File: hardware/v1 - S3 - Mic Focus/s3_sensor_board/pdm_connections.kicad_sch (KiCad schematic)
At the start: 2 parts, among them U501 SHT4x

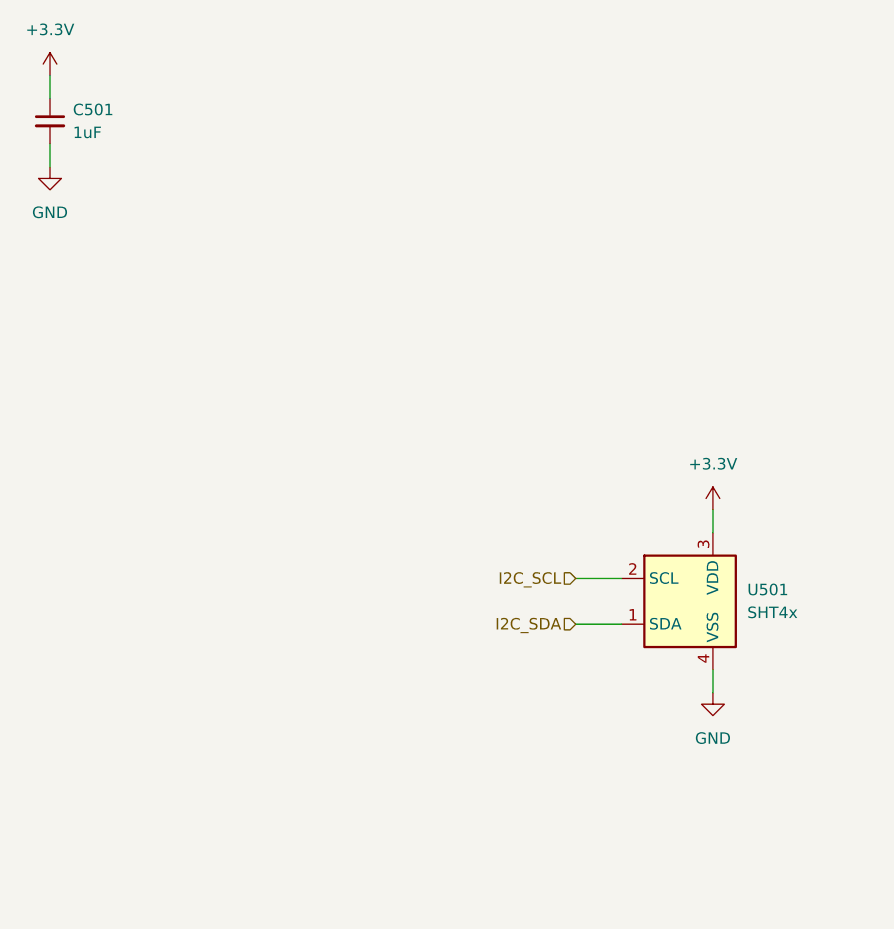
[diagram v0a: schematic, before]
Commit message: WIP
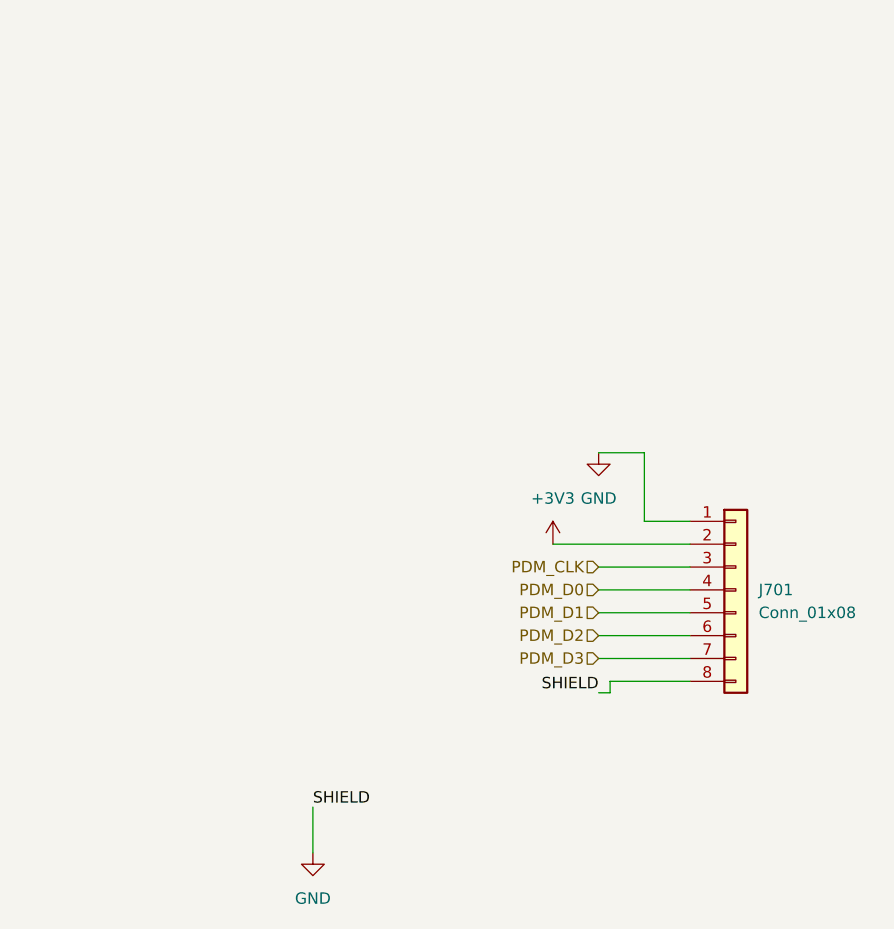
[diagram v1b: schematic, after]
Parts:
- removed C501: 1uF, Capacitor_SMD:C_0805_2012Metric, symbol Device:C_Small
- removed U501: SHT4x, Sensor_Humidity:Sensirion_DFN-4_1.5x1.5mm_P0.8mm_SHT4x_NoCentralPad, symbol Sensor_Humidity:SHT4x
- added J701: Conn_01x08, Connector_PinHeader_2.54mm:PinHeader_1x08_P2.54mm_Vertical, symbol Connector_Generic:Conn_01x08
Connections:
- net GND: now also J701.1 (Pin_1), J701.8 (Pin_8)
- new net +3V3: J701.2 (Pin_2)
- new net PDM_CLK: J701.3 (Pin_3)
- new net PDM_D0: J701.4 (Pin_4)
- new net PDM_D1: J701.5 (Pin_5)
- new net PDM_D2: J701.6 (Pin_6)
- new net PDM_D3: J701.7 (Pin_7)

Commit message: WIP
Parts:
- J701: footprint Connector_PinHeader_2.54mm:PinHeader_1x08_P2.54mm_Vertical -> Connector_IDC:IDC-Header_2x04_P2.54mm_Vertical
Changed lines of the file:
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@@
 			)
 		)
-		(property "Footprint" "Connector_PinHeader_2.54mm:PinHeader_1x08_P2.54mm_Vertical"
+		(property "Footprint" "Connector_IDC:IDC-Header_2x04_P2.54mm_Vertical"
 			(at 104.14 87.63 0)
 			(hide yes)
